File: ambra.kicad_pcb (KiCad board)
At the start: 2 copper layers, 129.8 x 99.4 mm, 34 parts, among them J1 MJ-4PP-9, SW1 SW_SPDT, U1 ProMicro_r

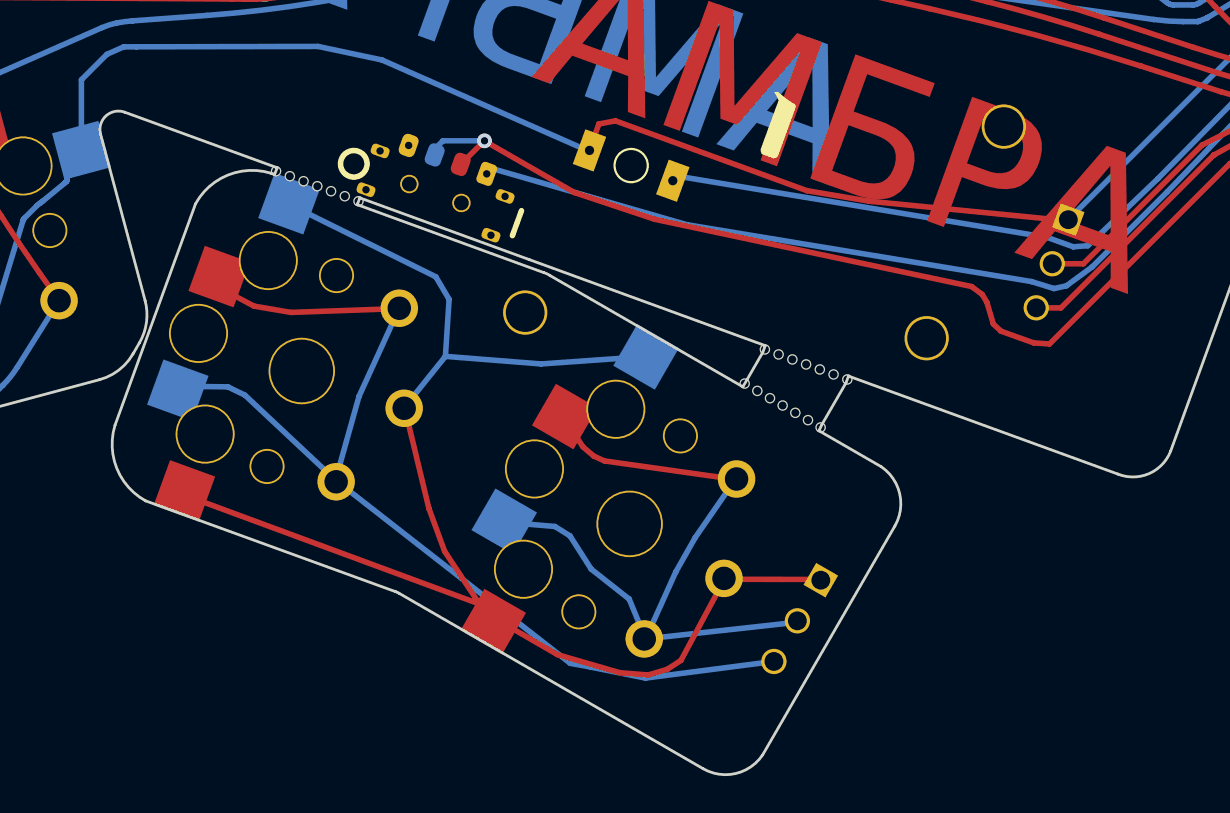
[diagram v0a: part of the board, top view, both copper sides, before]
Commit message: Add files via upload
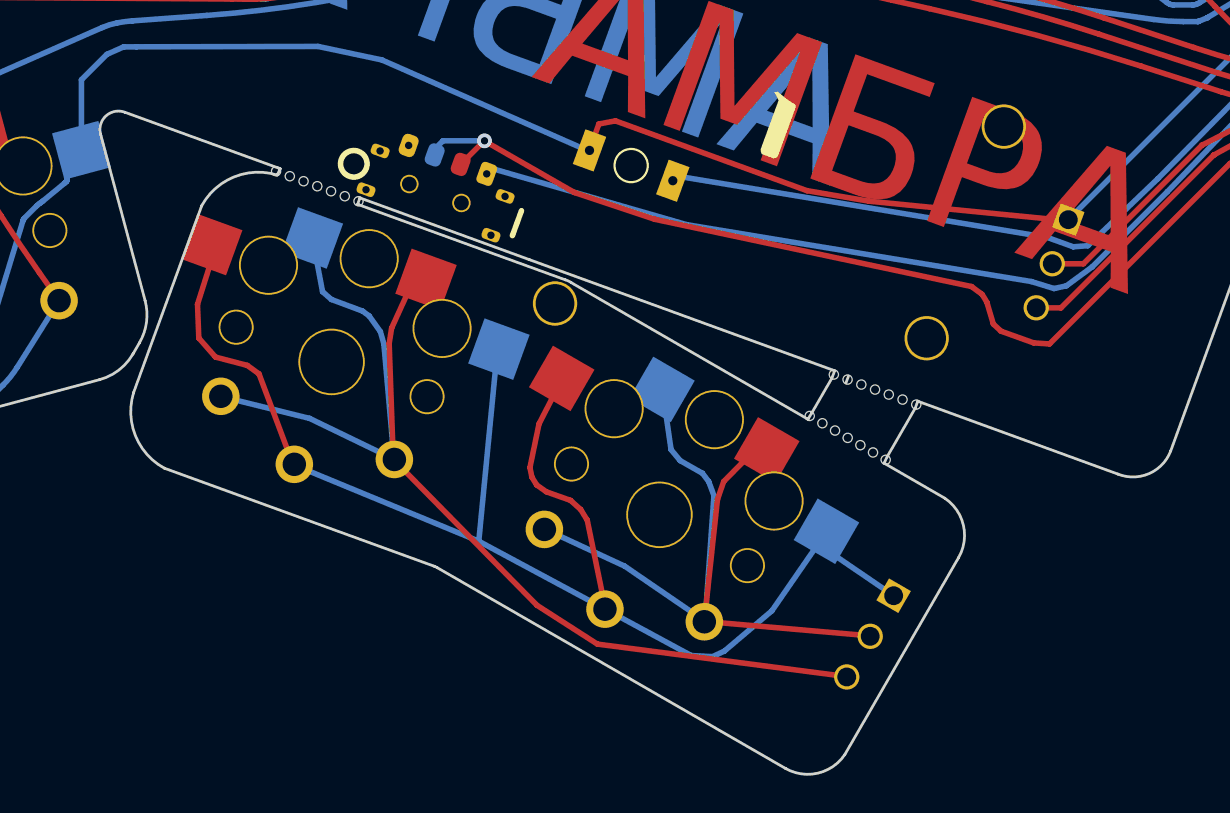
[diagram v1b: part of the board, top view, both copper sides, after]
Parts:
- moved REF** 4.03 mm to (162.0, 140.5)
- moved BT3 3.97 mm to (162.4, 127.1)
- moved BT3 3.93 mm to (160.9, 129.7)
- moved SWr4c2 1.69 mm to (132.9, 125.6), turned to -20 degrees
- moved H1 1.69 mm to (145.0, 122.4)
- moved SWr4c1 1.69 mm to (150.7, 133.9), turned to -30 degrees
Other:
- outline, holes or cut-outs redrawn

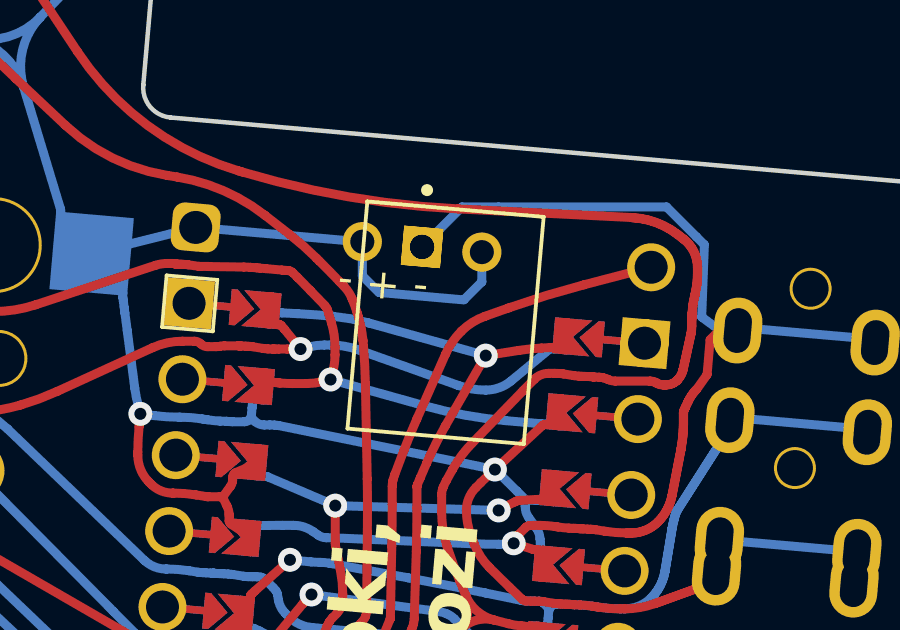
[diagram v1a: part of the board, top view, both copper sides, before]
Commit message: Add files via upload
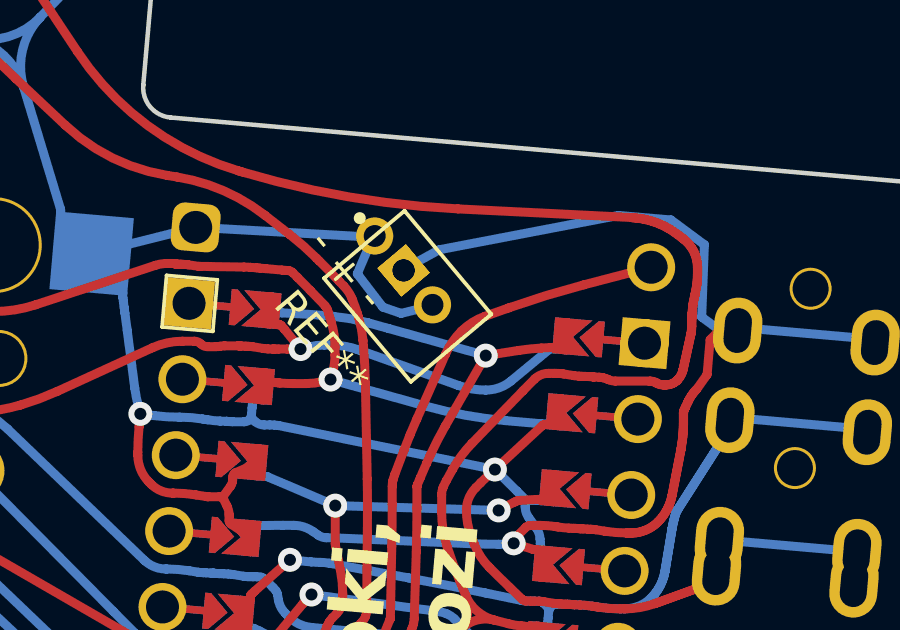
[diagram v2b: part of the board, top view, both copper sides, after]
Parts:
- removed the REF** at (206.4, 81.0)
- removed the REF** at (204.4, 80.9)
- added REF**: JST_B2B-ZR_LF__SN_, my syms-foots:JST_B2B-ZR_LF__SN_, F.Cu at (204.9, 82.6)
- added REF**: JST_B2B-ZR_LF__SN_, my syms-foots:JST_B2B-ZR_LF__SN_, B.Cu at (204.0, 81.5)
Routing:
- net VCC: track 42.1 -> 31.6 mm
- net GND: track 671.6 -> 667.8 mm
